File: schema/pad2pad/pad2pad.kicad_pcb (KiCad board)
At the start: 2 copper layers, 15.5 x 7.8 mm, 2 parts, among them J1 Conn_01x01_Male, J2 Conn_01x01_Male

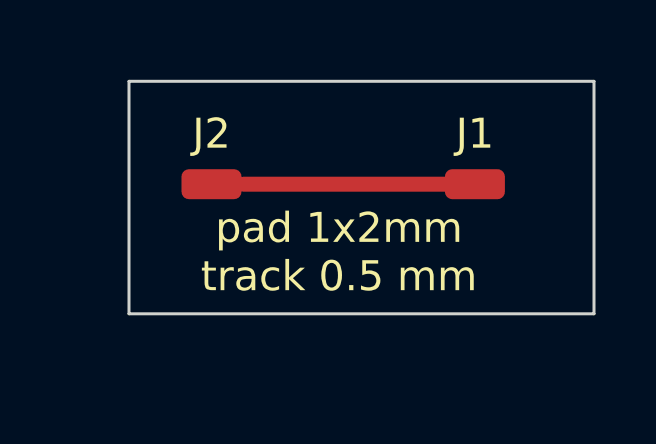
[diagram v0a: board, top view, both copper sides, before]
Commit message: ardrill command, pad2pad&soic projects
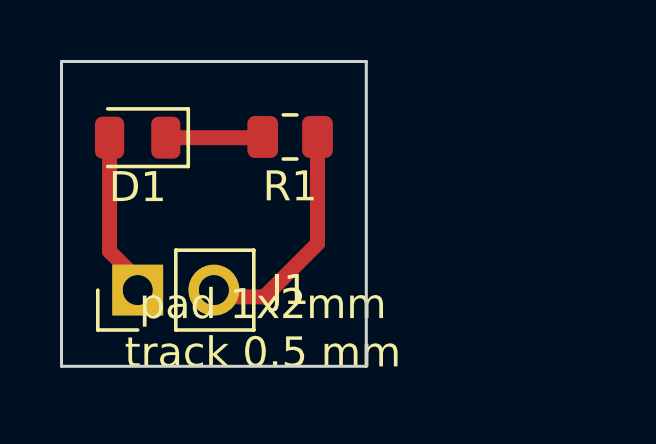
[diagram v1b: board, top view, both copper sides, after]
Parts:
- removed J2: Conn_01x01_Male, Connector_Wire:SolderWirePad_1x01_SMD_1x2mm
- added D1: LED, LED_SMD:LED_0805_2012Metric, F.Cu at (2.54, -7.62)
- added R1: R, Resistor_SMD:R_0805_2012Metric, F.Cu at (7.62, -7.64)
- J1: value Conn_01x01_Male -> Conn_01x02_Male; footprint Connector_Wire:SolderWirePad_1x01_SMD_1x2mm -> Connector_PinHeader_2.54mm:PinHeader_1x02_P2.54mm_Vertical
- moved J1 11.8 mm to (2.54, -2.54)
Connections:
- J1 pad 1: Net-(J1-Pad1) -> +5V
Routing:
- net Net-(J1-Pad1): track 7.71 -> 0.00 mm
- net GND: track 0.00 -> 7.36 mm
- net +5V: track 0.00 -> 5.22 mm
- net Net-(D1-Pad1): track 0.00 -> 2.97 mm
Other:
- board size 15.5 x 7.8 mm -> 10.2 x 10.2 mm
